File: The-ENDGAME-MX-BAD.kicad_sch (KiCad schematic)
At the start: 76 parts, among them J2 Conn_01x02_Female, SW1 SW_Push, SW10 SW_Push, SW11 SW_Push, SW12 SW_Push, SW13 SW_Push, SW14 SW_Push, SW15 SW_Push, SW16 SW_Push, SW17 SW_Push, SW18 SW_Push, SW19 SW_Push, SW2 SW_Push, SW20 SW_Push, SW21 SW_Push, SW22 SW_Push, SW23 SW_Push, SW24 SW_Push, SW25 SW_Push, SW26 SW_Push, SW27 SW_Push, SW28 SW_Push, SW29 SW_Push, SW3 SW_Push, SW30 SW_Push, SW31 SW_Push, SW32 SW_Push, SW33 SW_Push, SW34 SW_Push, SW35 SW_Push, SW36 SW_Push, SW4 SW_Push, SW5 SW_Push, SW6 SW_Push, SW7 SW_Push, SW8 SW_Push, SW9 SW_Push, U1 ProMicro-kbd-34key

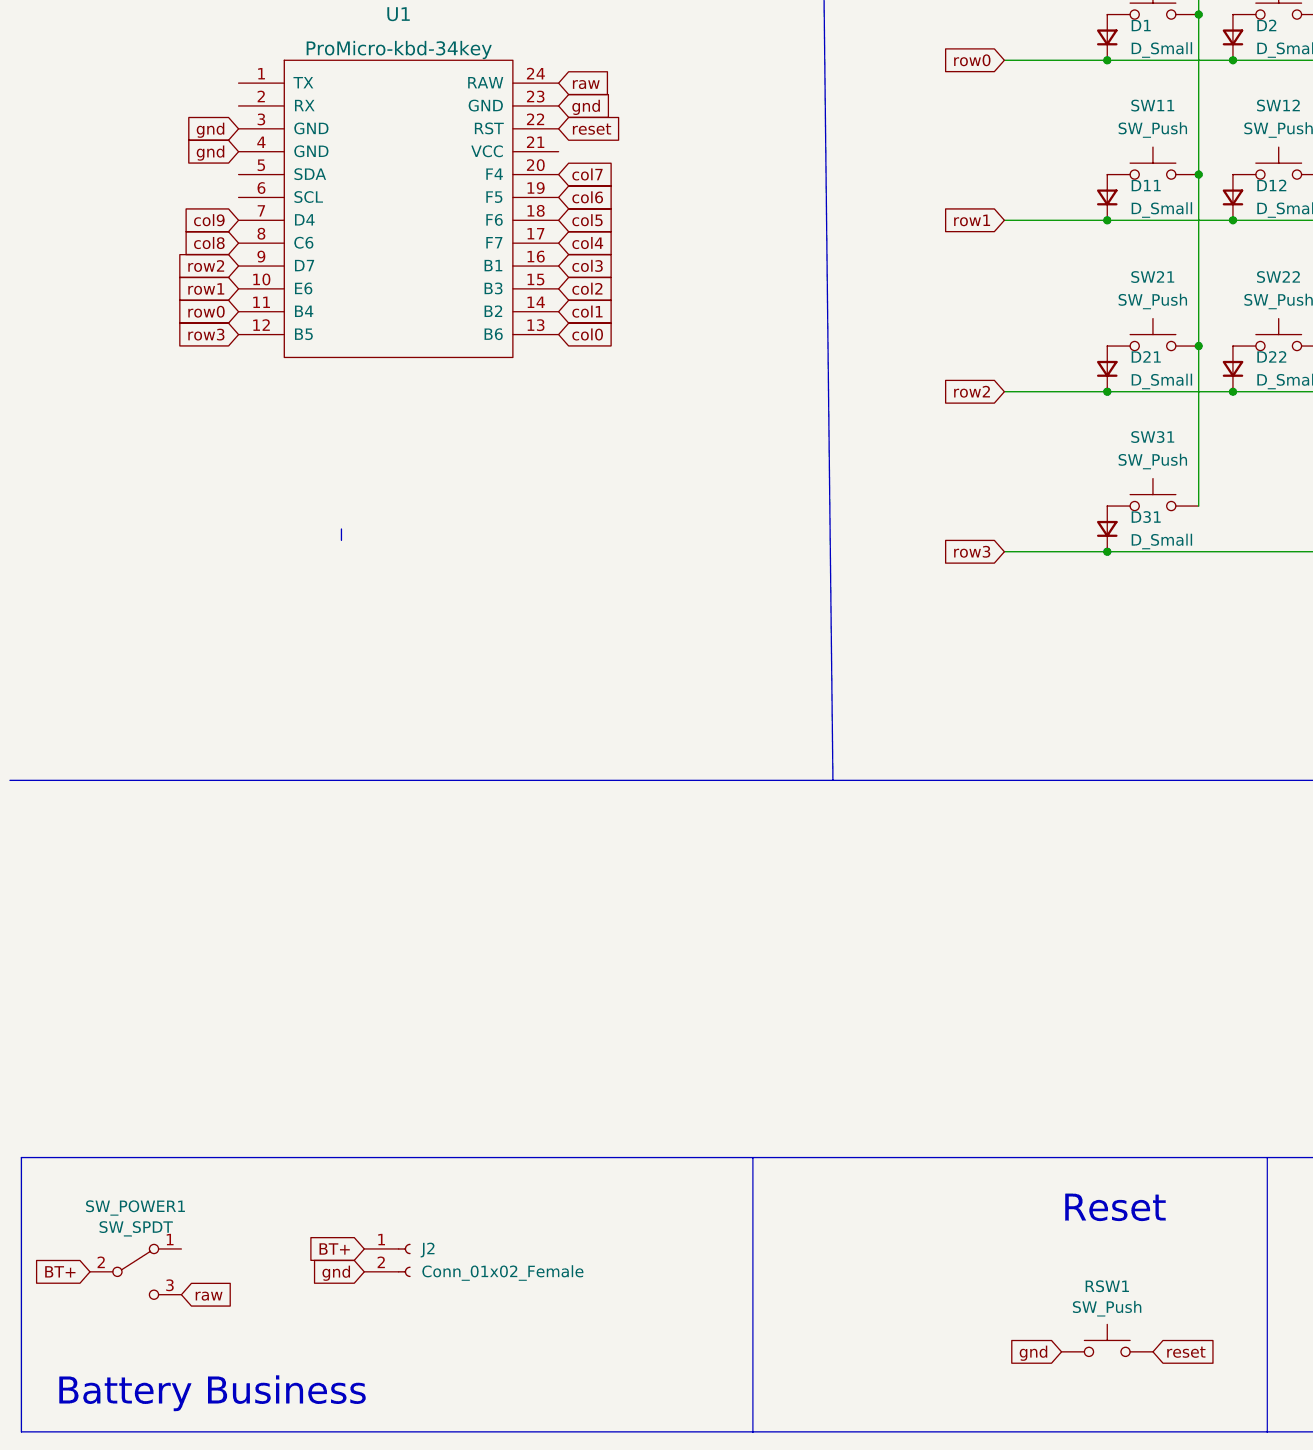
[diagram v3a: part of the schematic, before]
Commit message: updates updates upddfkjds
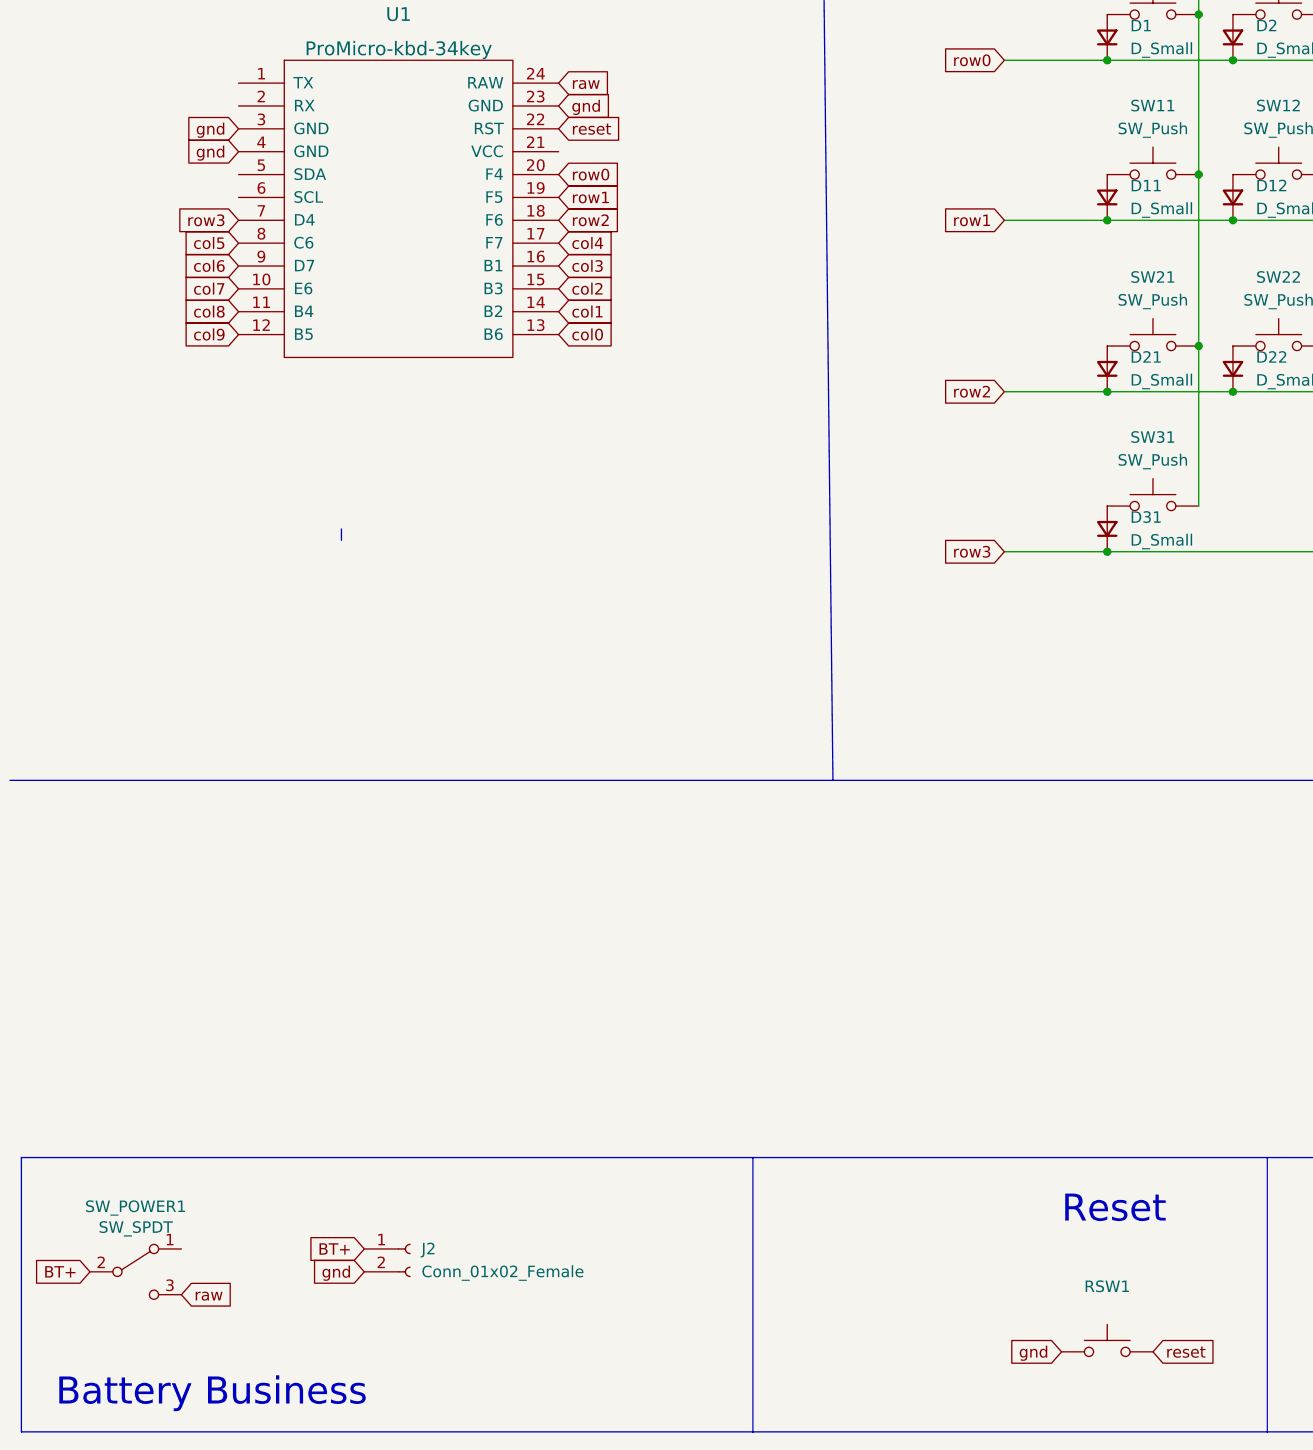
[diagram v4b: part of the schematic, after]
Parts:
- RSW1: value SW_Push -> (none); footprint Button_Switch_THT:SW_PUSH_6mm -> (none)
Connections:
- net col5: now also U1.8 (C6); no longer U1.18 (F6)
- net col6: now also U1.9 (D7); no longer U1.19 (F5)
- net col7: now also U1.10 (E6); no longer U1.20 (F4)
- net col8: now also U1.11 (B4); no longer U1.8 (C6)
- net col9: now also U1.12 (B5); no longer U1.7 (D4)
- net row0: now also U1.20 (F4); no longer U1.11 (B4)
- net row1: now also U1.19 (F5); no longer U1.10 (E6)
- net row2: now also U1.18 (F6); no longer U1.9 (D7)
- net row3: now also U1.7 (D4); no longer U1.12 (B5)
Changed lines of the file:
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@@
     )
   )
-  (global_label "col5" (shape input) (at 73.66 62.23 0) (fields_autoplaced)
-    (effects (font (size 1.27 1.27)) (justify left))
-    (property "Intersheet References" "${INTERSHEET_REFS}" (id 0) (at 80.1855 62.1506 0)
-      (effects (font (size 1.27 1.27)) (justify left) hide)
+  (global_label "col5" (shape input) (at 38.1 64.77 180) (fields_autoplaced)
+    (effects (font (size 1.27 1.27)) (justify right))
+    (property "Intersheet References" "${INTERSHEET_REFS}" (id 0) (at 31.5745 64.8494 0)
+      (effects (font (size 1.27 1.27)) (justify right) hide)
     )
   )
@@
     )
   )
-  (global_label "row1" (shape input) (at 38.1 69.85 180) (fields_autoplaced)
+  (global_label "row1" (shape input) (at 73.66 59.69 0) (fields_autoplaced)
+    (effects (font (size 1.27 1.27)) (justify left))
+    (property "Intersheet References" "${INTERSHEET_REFS}" (id 0) (at 80.5483 59.7694 0)
+      (effects (font (size 1.27 1.27)) (justify left) hide)
+    )
+  )
+  (global_label "col1" (shape input) (at 158.75 21.59 90) (fields_autoplaced)
+    (effects (font (size 1.27 1.27)) (justify left))
+    (property "Intersheet References" "${INTERSHEET_REFS}" (id 0) (at 158.6706 15.0645 90)
+      (effects (font (size 1.27 1.27)) (justify left) hide)
+    )
+  )
+  (global_label "row3" (shape input) (at 38.1 62.23 180) (fields_autoplaced)
     (effects (font (size 1.27 1.27)) (justify right))
-    (property "Intersheet References" "${INTERSHEET_REFS}" (id 0) (at 31.2117 69.7706 0)
+    (property "Intersheet References" "${INTERSHEET_REFS}" (id 0) (at 31.2117 62.1506 0)
       (effects (font (size 1.27 1.27)) (justify right) hide)
     )
   )
-  (global_label "col1" (shape input) (at 158.75 21.59 90) (fields_autoplaced)
-    (effects (font (size 1.27 1.27)) (justify left))
-    (property "Intersheet References" "${INTERSHEET_REFS}" (id 0) (at 158.6706 15.0645 90)
-      (effects (font (size 1.27 1.27)) (justify left) hide)
-    )
-  )
-  (global_label "row3" (shape input) (at 38.1 74.93 180) (fields_autoplaced)
+  (global_label "raw" (shape input) (at 31.75 181.61 0) (fields_autoplaced)
+    (effects (font (size 1.27 1.27)) (justify left))
+    (property "Intersheet References" "${INTERSHEET_REFS}" (id 0) (at -16.51 405.13 0)
+      (effects (font (size 1.27 1.27)) hide)
+    )
+  )
+  (global_label "col7" (shape input) (at 38.1 69.85 180) (fields_autoplaced)
     (effects (font (size 1.27 1.27)) (justify right))
-    (property "Intersheet References" "${INTERSHEET_REFS}" (id 0) (at 31.2117 74.8506 0)
+    (property "Intersheet References" "${INTERSHEET_REFS}" (id 0) (at 31.5745 69.9294 0)
       (effects (font (size 1.27 1.27)) (justify right) hide)
     )
   )
-  (global_label "raw" (shape input) (at 31.75 181.61 0) (fields_autoplaced)
-    (effects (font (size 1.27 1.27)) (justify left))
-    (property "Intersheet References" "${INTERSHEET_REFS}" (id 0) (at -16.51 405.13 0)
-      (effects (font (size 1.27 1.27)) hide)
-    )
-  )
-  (global_label "col7" (shape input) (at 73.66 57.15 0) (fields_autoplaced)
-    (effects (font (size 1.27 1.27)) (justify left))
-    (property "Intersheet References" "${INTERSHEET_REFS}" (id 0) (at 80.1855 57.0706 0)
-      (effects (font (size 1.27 1.27)) (justify left) hide)
-    )
-  )
-  (global_label "row2" (shape input) (at 38.1 67.31 180) (fields_autoplaced)
-    (effects (font (size 1.27 1.27)) (justify right))
-    (property "Intersheet References" "${INTERSHEET_REFS}" (id 0) (at 31.2117 67.2306 0)
-      (effects (font (size 1.27 1.27)) (justify right) hide)
+  (global_label "row2" (shape input) (at 73.66 62.23 0) (fields_autoplaced)
+    (effects (font (size 1.27 1.27)) (justify left))
+    (property "Intersheet References" "${INTERSHEET_REFS}" (id 0) (at 80.5483 62.3094 0)
+      (effects (font (size 1.27 1.27)) (justify left) hide)
     )
   )
@@
     )
   )
-  (global_label "col6" (shape input) (at 73.66 59.69 0) (fields_autoplaced)
-    (effects (font (size 1.27 1.27)) (justify left))
-    (property "Intersheet References" "${INTERSHEET_REFS}" (id 0) (at 80.1855 59.6106 0)
-      (effects (font (size 1.27 1.27)) (justify left) hide)
+  (global_label "col6" (shape input) (at 38.1 67.31 180) (fields_autoplaced)
+    (effects (font (size 1.27 1.27)) (justify right))
+    (property "Intersheet References" "${INTERSHEET_REFS}" (id 0) (at 31.5745 67.3894 0)
+      (effects (font (size 1.27 1.27)) (justify right) hide)
     )
   )
@@
     )
   )
-  (global_label "row0" (shape input) (at 38.1 72.39 180) (fields_autoplaced)
+  (global_label "row0" (shape input) (at 73.66 57.15 0) (fields_autoplaced)
+    (effects (font (size 1.27 1.27)) (justify left))
+    (property "Intersheet References" "${INTERSHEET_REFS}" (id 0) (at 80.5483 57.2294 0)
+      (effects (font (size 1.27 1.27)) (justify left) hide)
+    )
+  )
+  (global_label "col8" (shape input) (at 256.54 21.59 90) (fields_autoplaced)
+    (effects (font (size 1.27 1.27)) (justify left))
+    (property "Intersheet References" "${INTERSHEET_REFS}" (id 0) (at 256.4606 15.0645 90)
+      (effects (font (size 1.27 1.27)) (justify left) hide)
+    )
+  )
+  (global_label "col4" (shape input) (at 200.66 21.59 90) (fields_autoplaced)
+    (effects (font (size 1.27 1.27)) (justify left))
+    (property "Intersheet References" "${INTERSHEET_REFS}" (id 0) (at 200.5806 15.0645 90)
+      (effects (font (size 1.27 1.27)) (justify left) hide)
+    )
+  )
+  (global_label "col0" (shape input) (at 73.66 74.93 0) (fields_autoplaced)
+    (effects (font (size 1.27 1.27)) (justify left))
+    (property "Intersheet References" "${INTERSHEET_REFS}" (id 0) (at 80.1855 74.8506 0)
+      (effects (font (size 1.27 1.27)) (justify left) hide)
+    )
+  )
+  (global_label "col8" (shape input) (at 38.1 72.39 180) (fields_autoplaced)
     (effects (font (size 1.27 1.27)) (justify right))
-    (property "Intersheet References" "${INTERSHEET_REFS}" (id 0) (at 31.2117 72.3106 0)
-      (effects (font (size 1.27 1.27)) (justify right) hide)
-    )
-  )
-  (global_label "col8" (shape input) (at 256.54 21.59 90) (fields_autoplaced)
-    (effects (font (size 1.27 1.27)) (justify left))
-    (property "Intersheet References" "${INTERSHEET_REFS}" (id 0) (at 256.4606 15.0645 90)
-      (effects (font (size 1.27 1.27)) (justify left) hide)
-    )
-  )
-  (global_label "col4" (shape input) (at 200.66 21.59 90) (fields_autoplaced)
-    (effects (font (size 1.27 1.27)) (justify left))
-    (property "Intersheet References" "${INTERSHEET_REFS}" (id 0) (at 200.5806 15.0645 90)
-      (effects (font (size 1.27 1.27)) (justify left) hide)
-    )
-  )
-  (global_label "col0" (shape input) (at 73.66 74.93 0) (fields_autoplaced)
-    (effects (font (size 1.27 1.27)) (justify left))
-    (property "Intersheet References" "${INTERSHEET_REFS}" (id 0) (at 80.1855 74.8506 0)
-      (effects (font (size 1.27 1.27)) (justify left) hide)
-    )
-  )
-  (global_label "col8" (shape input) (at 38.1 64.77 180) (fields_autoplaced)
-    (effects (font (size 1.27 1.27)) (justify right))
-    (property "Intersheet References" "${INTERSHEET_REFS}" (id 0) (at 31.5745 64.8494 0)
+    (property "Intersheet References" "${INTERSHEET_REFS}" (id 0) (at 31.5745 72.4694 0)
       (effects (font (size 1.27 1.27)) (justify right) hide)
     )
@@
     )
   )
-  (global_label "col9" (shape input) (at 38.1 62.23 180) (fields_autoplaced)
+  (global_label "col9" (shape input) (at 38.1 74.93 180) (fields_autoplaced)
     (effects (font (size 1.27 1.27)) (justify right))
-    (property "Intersheet References" "${INTERSHEET_REFS}" (id 0) (at 31.5745 62.3094 0)
+    (property "Intersheet References" "${INTERSHEET_REFS}" (id 0) (at 31.5745 75.0094 0)
       (effects (font (size 1.27 1.27)) (justify right) hide)
     )
@@
     (in_bom yes) (on_board yes)
     (property "Reference" "RSW1" (id 0) (at 134.62 180.721 0))
-    (property "Value" "SW_Push" (id 1) (at 134.62 183.0324 0))
-    (property "Footprint" "Button_Switch_THT:SW_PUSH_6mm" (id 2) (at 134.62 182.88 0)
+    (property "Value" "" (id 1) (at 134.62 183.0324 0))
+    (property "Footprint" "" (id 2) (at 134.62 182.88 0)
       (effects (font (size 1.27 1.27)) hide)
     )
@@
     )
     (path "/8c098b2f-e56b-4cd0-858f-8acf9e4a45b2"
-      (reference "RSW1") (unit 1) (value "SW_Push") (footprint "Button_Switch_THT:SW_PUSH_6mm")
+      (reference "RSW1") (unit 1) (value "SW_Push") (footprint "Button_Switch_SMD:SW_SPST_TL3342")
     )
     (path "/c072b47f-dc52-4968-be95-dfa9d02b31ad"
